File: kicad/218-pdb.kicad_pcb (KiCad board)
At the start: 2 copper layers, 80 x 55.4 mm, 73 parts, among them J1 Conn_01x03, J10 Conn_01x03, J11 Conn_01x03, J12 Conn_01x03, J13 Conn_01x03, J14 Conn_01x03, J15 Conn_01x03, J16 Conn_01x03, J17 Conn_01x03, J18 Conn_01x03, J19 Conn_01x03, J2 Conn_01x03, J20 Conn_01x03, J21 Conn_01x03, J22 Conn_01x03, J23 Conn_01x03, J24 Conn_01x03, J25 Conn_01x04_Pin, J26 Conn_01x04_Pin, J27 Conn_01x04_Pin, J28 Conn_01x04_Pin, J29 14 V molex, J3 Conn_01x03, J30 14 V molex, J31 14 V molex, J32 14 V molex, J33 external 5V, J34 battery, J35 battery, J4 Conn_01x03, J5 Conn_01x03, J6 Conn_01x03, J7 Conn_01x03, J8 Conn_01x03, J9 Conn_01x03, SW1 5V switch, U1 DC-DC buck, U2 DC-DC buck, U3 LD1117V33, U4 LD1117V33

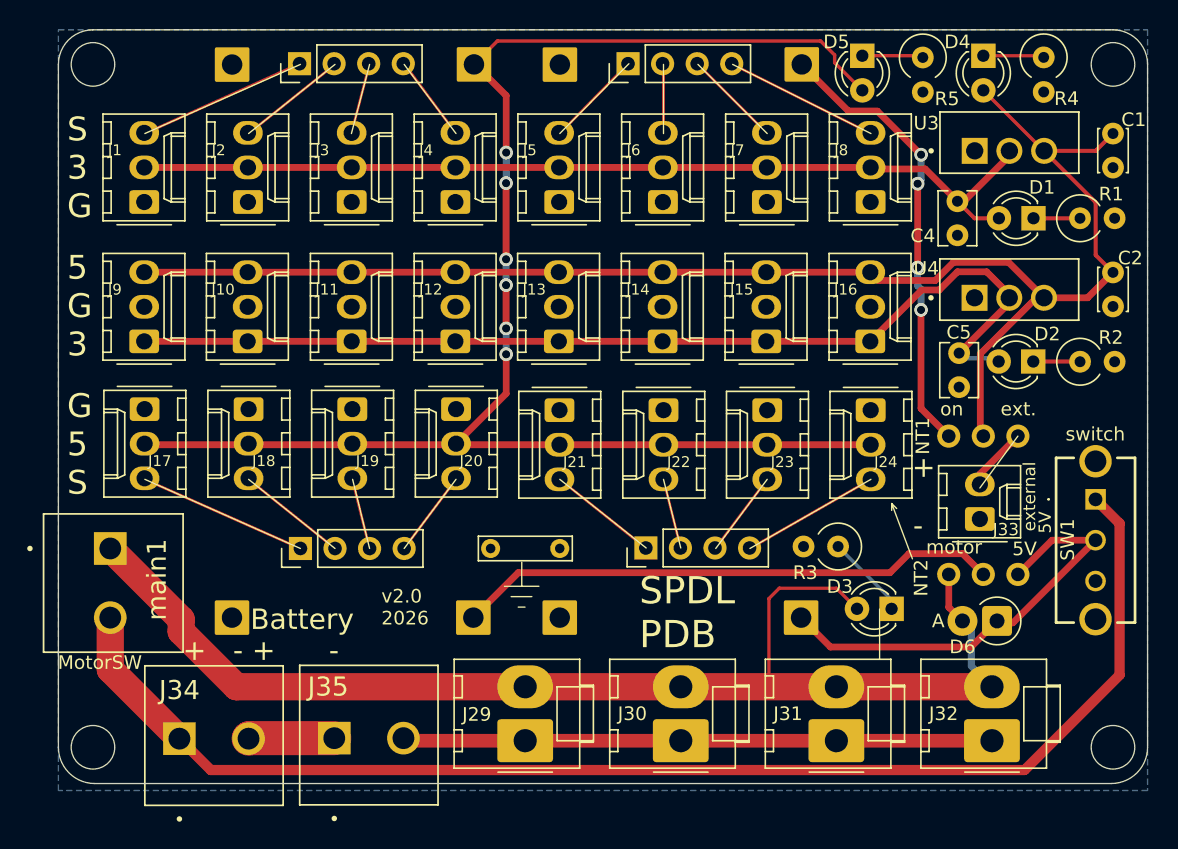
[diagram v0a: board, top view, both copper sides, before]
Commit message: update script
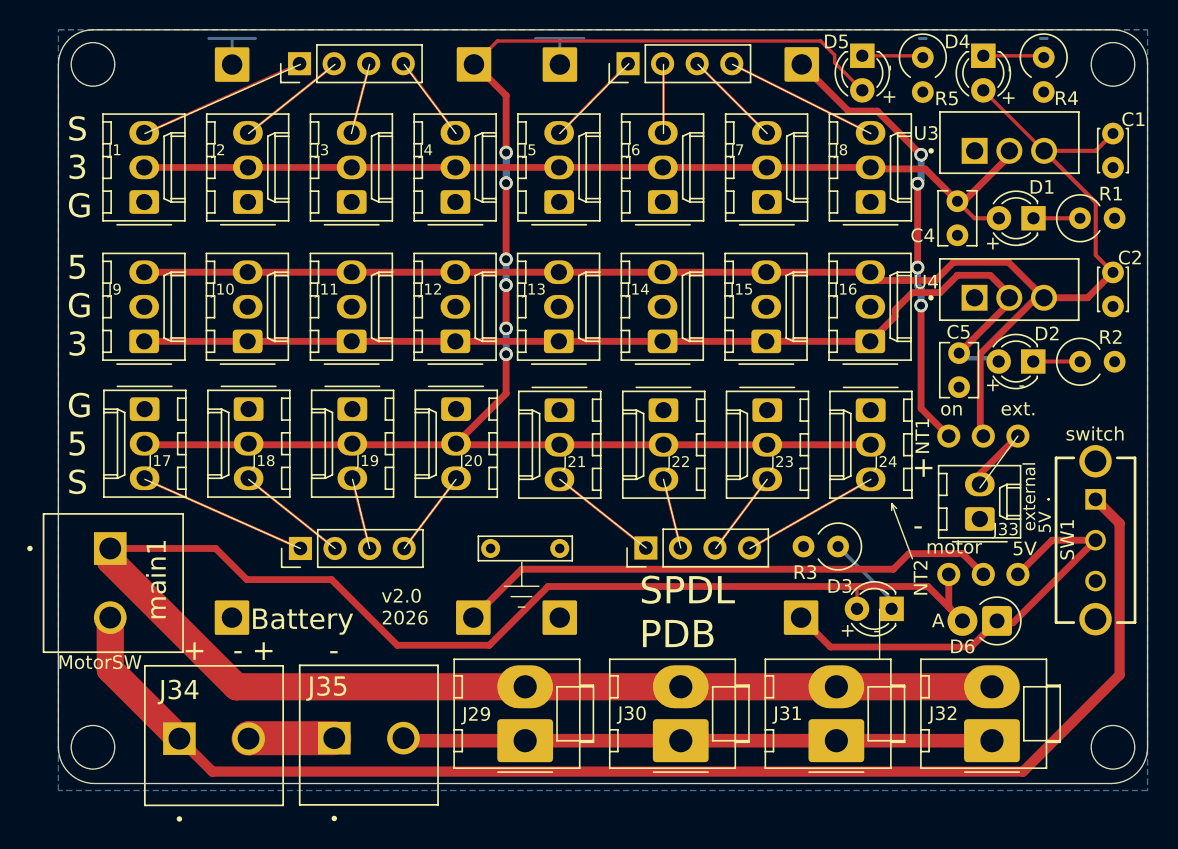
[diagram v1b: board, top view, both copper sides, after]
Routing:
- net 14-3: track 97.9 -> 143.4 mm
- net GND: track 43.3 -> 54.2 mm
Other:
- board text added: "+ -"
